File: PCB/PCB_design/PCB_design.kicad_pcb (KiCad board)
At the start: 2 copper layers, 68.2 x 66 mm, 55 parts, among them J1 Conn_01x01_Pin, J2 Conn_01x01_Pin, J3 Conn_01x01_Pin, J4 Conn_01x01_Pin, J5 Conn_01x01_Pin, J6 Conn_01x01_Pin, J7 Conn_02x04_Counter_Clockwise, J8 Conn_01x01_Pin, K1 Relay_SPST-NO, K2 Relay_SPST-NO, K3 Relay_SPST-NO, K4 Relay_SPST-NO, Q1 MMBT3904, Q2 MMBT3904, Q3 MMBT3904, Q4 MMBT3904, T1 Transformer_1P_2S, U1 SCJT1117B-3.3-A

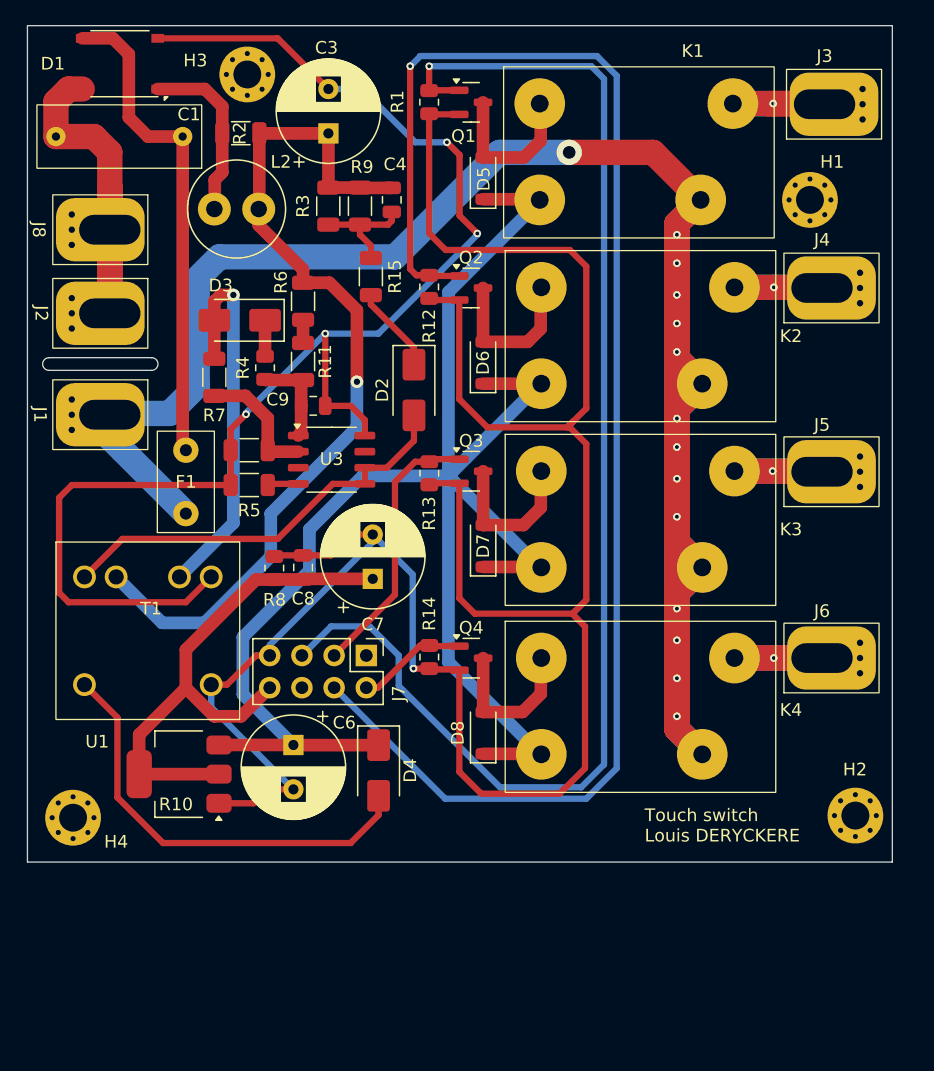
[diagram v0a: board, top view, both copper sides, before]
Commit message: Regroupement partie AC
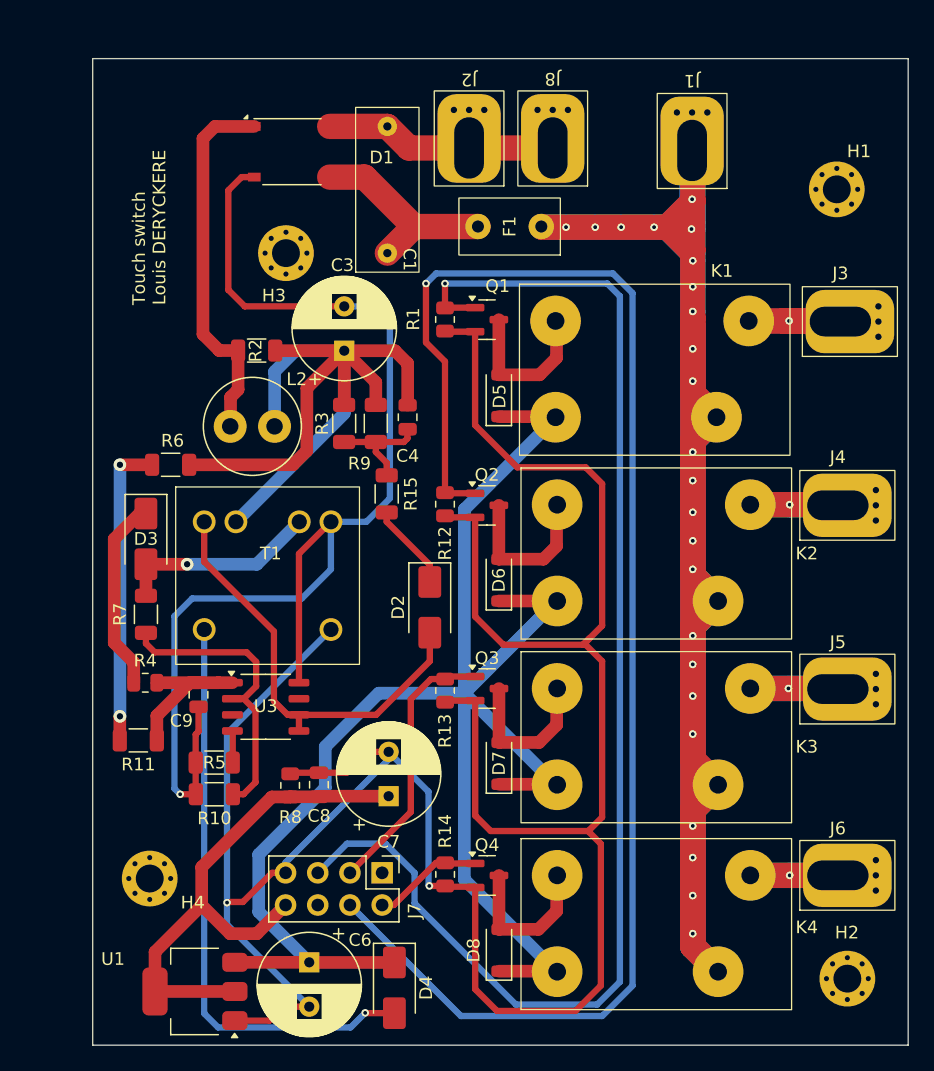
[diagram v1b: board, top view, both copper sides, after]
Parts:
- moved J1 50.5 mm to (145.9, 37.9), turned to 180 degrees
- moved J8 35.5 mm to (134.9, 37.6), turned to 180 degrees
- moved R11 32.6 mm to (102.2, 84.4), turned to 0 degrees
- moved F1 32.5 mm to (131.6, 43.9), turned to 180 degrees
- moved J2 31.2 mm to (128.3, 37.6), turned to 180 degrees
- moved R10 27.3 mm to (108.2, 88.7)
- moved R4 26.6 mm to (102.8, 79.8), turned to 180 degrees
- moved C9 24.5 mm to (107.0, 80.8), turned to -90 degrees
- moved R5 22.1 mm to (108.2, 86.2)
- moved U3 20.2 mm to (112.3, 81.8)
- moved R7 19.5 mm to (102.8, 74.5)
- moved D3 18.8 mm to (102.8, 68.5), turned to -90 degrees
- moved C1 18.6 mm to (121.9, 46.0), turned to 90 degrees
- moved C8 17.2 mm to (116.5, 87.9)
- moved D2 17.2 mm to (125.2, 73.9)
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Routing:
- net L: track 251.2 -> 279.2 mm, vias 14 -> 24
- net N: track 41.3 -> 18.3 mm
- net Net-(C1-Pad1): track 38.9 -> 16.3 mm
- net Net-(R11-Pad1): track 1.83 -> 24.3 mm, vias 0 -> 2
- net GND2: track 187.6 -> 208.9 mm, vias 1 -> 2
- net Net-(D1-+): track 14.3 -> 29.7 mm
- net Vaux: track 30.3 -> 16.0 mm
- net Net-(U3-FB): track 9.94 -> 23.5 mm
- net GND: track 109.9 -> 97.2 mm, vias 4 -> 1
- net Net-(D3-K): track 2.84 -> 15.3 mm
- net Net-(D4-A): track 34.5 -> 46.2 mm, vias 0 -> 1
- net VCC_IC: track 7.56 -> 12.3 mm
- net C: track 33.2 -> 34.5 mm
- net +310VDC: track 71.8 -> 70.7 mm, vias 1 -> 0
- net CT2: track 118.9 -> 118.4 mm
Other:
- board size 68.2 x 66 mm -> 64.3 x 77.8 mm
